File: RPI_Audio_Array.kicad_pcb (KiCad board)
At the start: 2 copper layers, 57 parts, among them J1 Conn_02x20_Odd_Even, U1 PCMD3140IRTER, U2 SPH0690LM4H-1, U3 SPH0690LM4H-1, U4 SPH0690LM4H-1, U5 SPH0690LM4H-1, U6 TLV7103318QDSERQ1

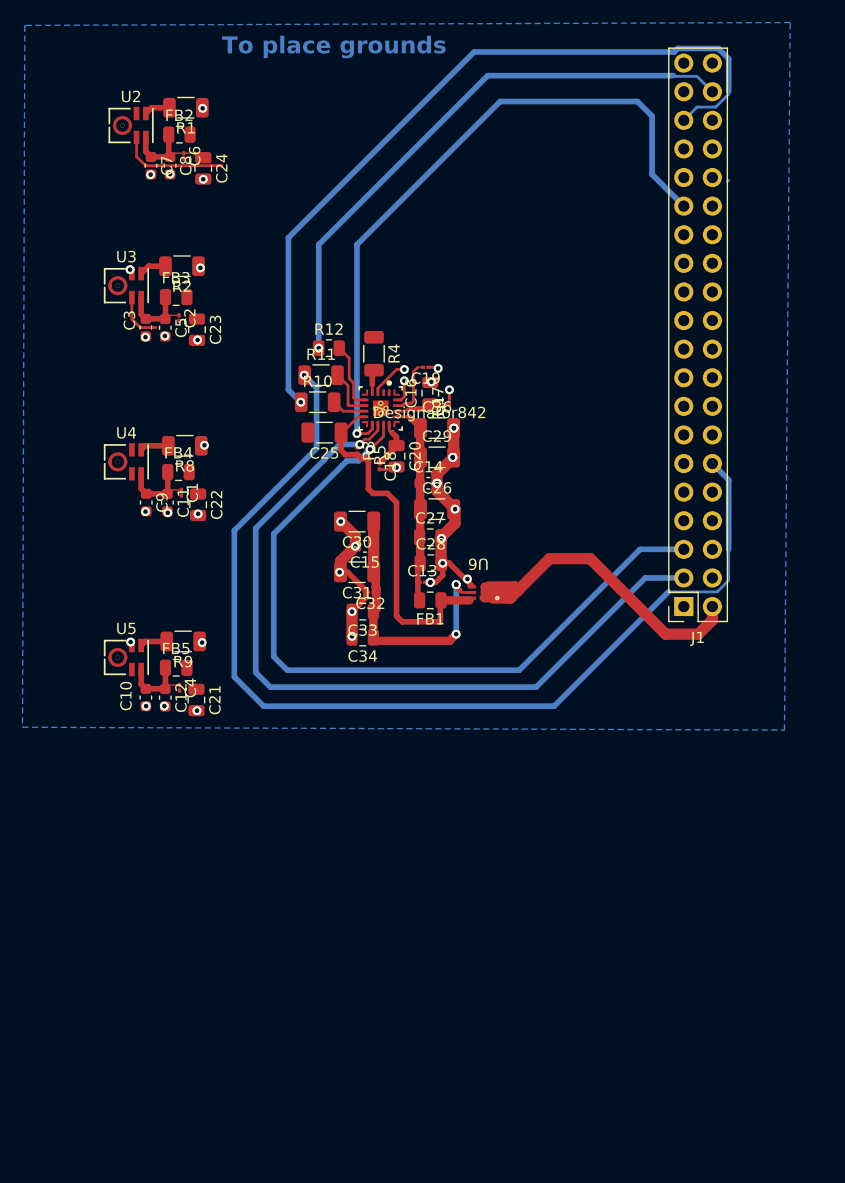
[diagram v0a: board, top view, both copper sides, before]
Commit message: Feat: adding more routing
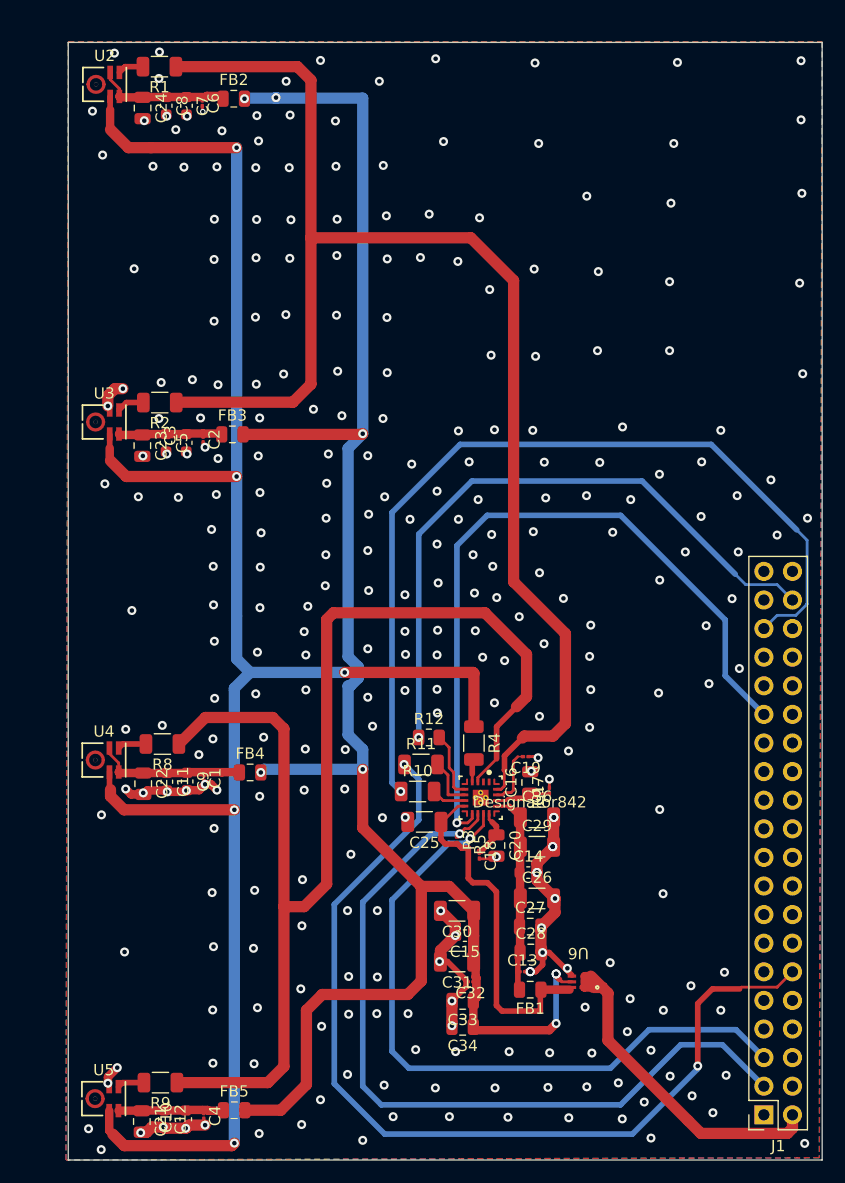
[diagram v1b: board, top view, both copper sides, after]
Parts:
- moved J1 45.7 mm to (90.4, 121.3)
- moved FB5 39.6 mm to (43.4, 120.9)
- moved R9 39.2 mm to (36.8, 118.4)
- moved U5 39.2 mm to (31.8, 119.8)
- moved C4 38.1 mm to (40.7, 121.4)
- moved C21 37.7 mm to (35.2, 121.9)
- moved C10 37.6 mm to (39.1, 121.7)
- moved C12 37.4 mm to (37.2, 121.7)
- moved C15 35.7 mm to (63.9, 105.4)
- moved C17 35.7 mm to (71.4, 92.5)
- moved C20 35.7 mm to (66.7, 97.4)
- moved C30 35.7 mm to (63.2, 103.2)
- moved C31 35.7 mm to (63.2, 107.7)
- moved C33 35.7 mm to (63.7, 111.2)
- moved FB1 35.7 mm to (69.7, 110.2)
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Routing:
- net PDMCLK: track 13.9 -> 170.4 mm, vias 0 -> 5
- net FILTER_BANK_1: track 28.0 -> 170.7 mm, vias 3 -> 8
- net PDM_IN_2: track 2.99 -> 123.5 mm, vias 3 -> 0
- net PDM_IN_1: track 3.76 -> 111.6 mm, vias 3 -> 0
- net GND: track 37.9 -> 59.8 mm, vias 35 -> 291
- net FSYNC: track 69.6 -> 78.4 mm
- net FBCLK: track 90.9 -> 83.9 mm, vias 1 -> 2
- net SELECT_1: track 7.18 -> 13.9 mm
- net SDOUT: track 51.0 -> 57.6 mm
- net SCL: track 67.2 -> 62.0 mm
- net PCMD_GPIO1: track 60.1 -> 65.2 mm
- net SELECT_2: track 9.25 -> 12.3 mm
- net Net-(U3-VDD): track 7.10 -> 9.52 mm
- net Net-(U5-VDD): track 7.49 -> 9.87 mm
- net +5V: track 35.1 -> 33.3 mm
- added copper zone on F.Cu, net GND
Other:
- board outline added: 66.9 x 99.2 mm
- board text removed: "To place grounds"
